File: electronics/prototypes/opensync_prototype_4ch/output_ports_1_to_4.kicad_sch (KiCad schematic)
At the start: 24 parts, among them J4 61611042121502, J5 61611042121502, J6 61611042121502, J7 61611042121502, U5 SN74LVC1T45DCKR, U6 SN74LVC1T45DCKR, U7 SN74LVC1T45DCKR, U8 SN74LVC1T45DCKR

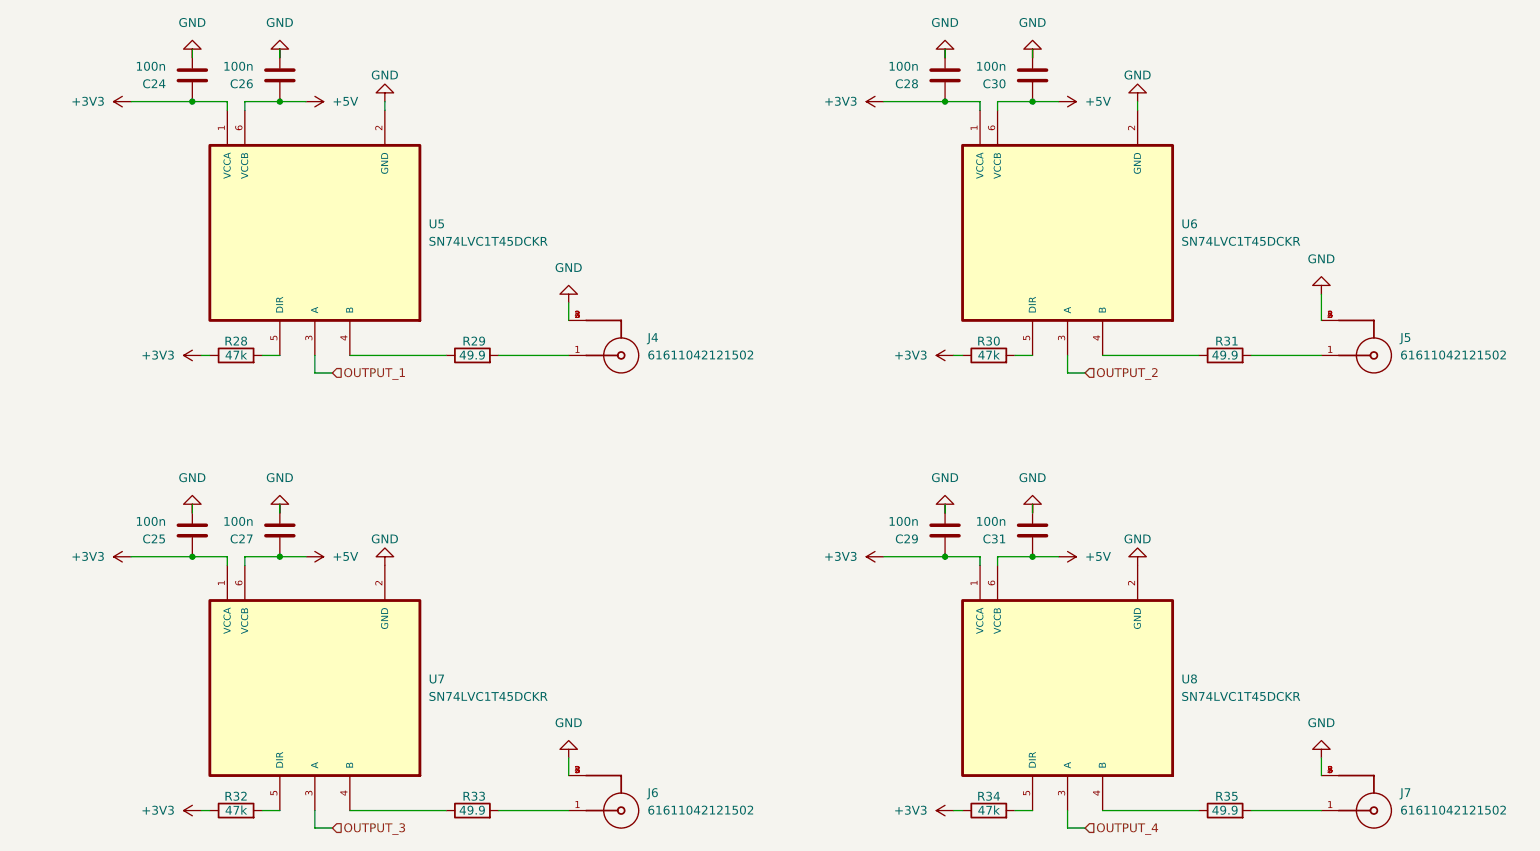
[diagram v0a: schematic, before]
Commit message: More prototyping
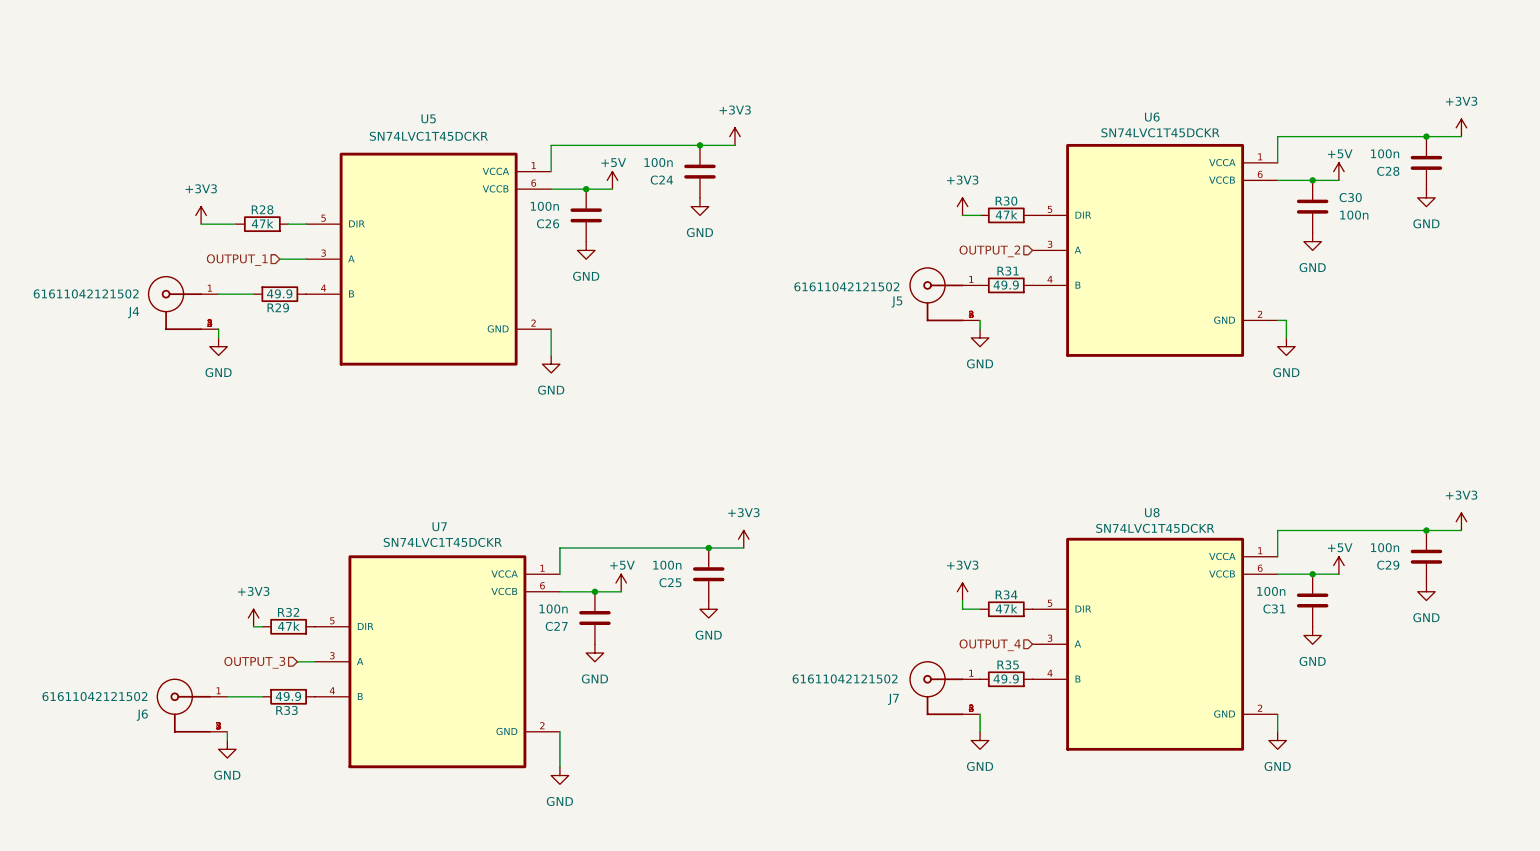
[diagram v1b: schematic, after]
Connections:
- net +3V3: now also C24.2, C25.2, C28.2, C29.2; no longer C24.1, C25.1, C28.1, C29.1
- net +5V: now also C26.2, C27.2, C31.2; no longer C26.1, C27.1, C31.1
- net GND: now also C24.1, C25.1, C26.1, C27.1, C28.1, C29.1, C31.1; no longer C24.2, C25.2, C26.2, C27.2, C28.2, C29.2, C31.2
- net at R35.1: now also J7.1; no longer U8.4 (B)
- net at R35.2: now also U8.4 (B); no longer J7.1
- net at R31.1: now also J5.1; no longer U6.4 (B)
- net at R31.2: now also U6.4 (B); no longer J5.1
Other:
- moved on the sheet: C24, C25, C26, C27, C28, C29, C30, C31, J4, J5, J6, J7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
